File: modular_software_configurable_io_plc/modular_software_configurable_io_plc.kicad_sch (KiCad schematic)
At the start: 8 parts, among them J1 FW-14-03-G-D-085-315, J2 FW-02-03-G-D-085-315, J3 FW-02-03-G-D-085-315, J4 FW-04-03-G-D-085-315, J5 FW-04-03-G-D-085-315, J6 FW-02-03-G-D-085-315, J7 FW-02-03-G-D-085-315, J8 FW-14-03-G-D-085-315

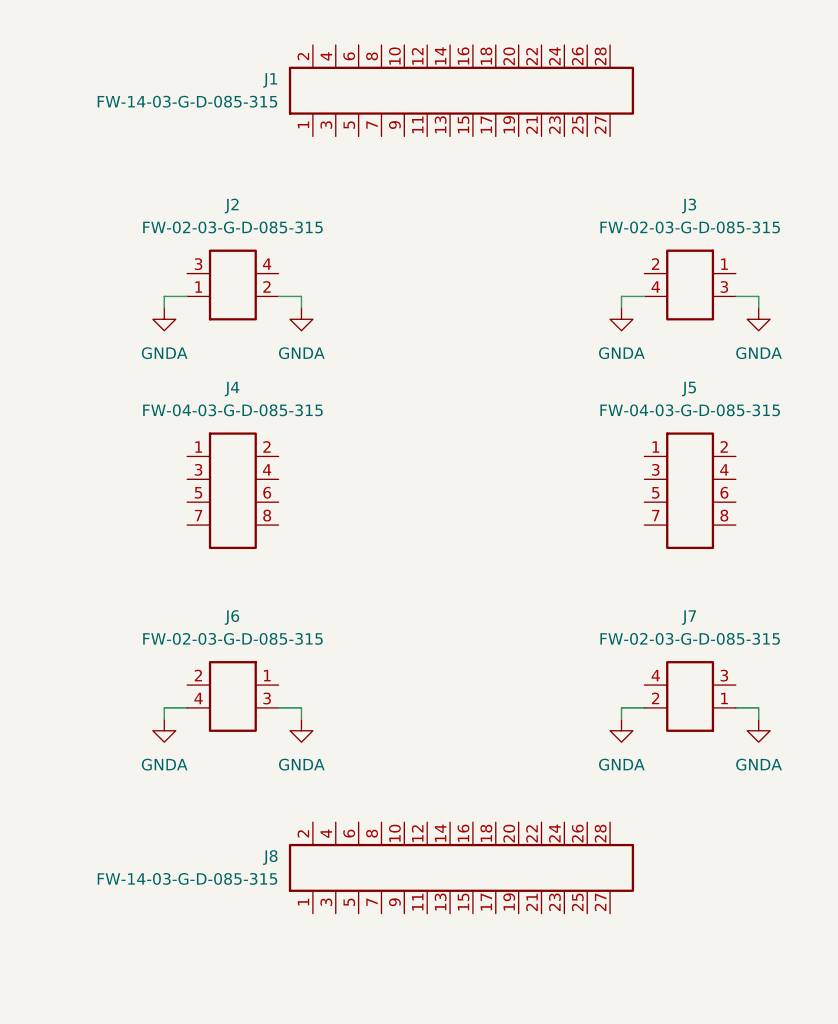
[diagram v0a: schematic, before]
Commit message: Minor updates to project files
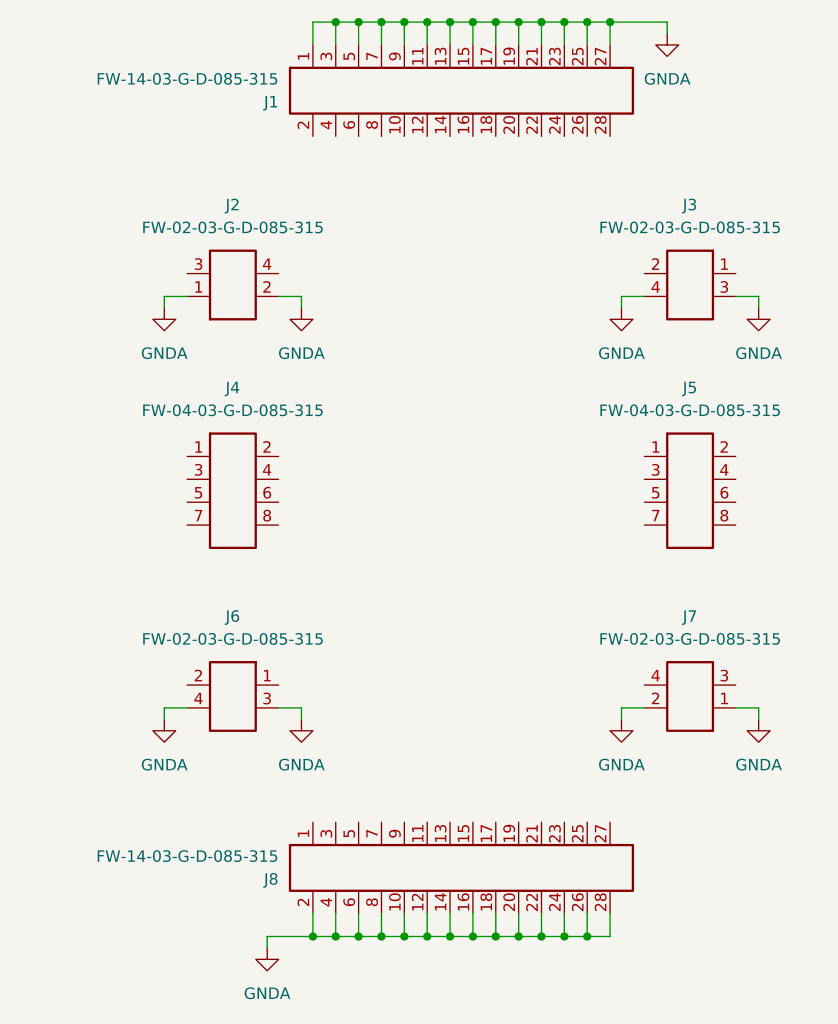
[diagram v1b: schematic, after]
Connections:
- net GNDA: now also J1.1, J1.11, J1.13, J1.15, J1.17, J1.19, J1.21, J1.23, J1.25, J1.27, J1.3, J1.5, J1.7, J1.9, J8.10, J8.12, J8.14, J8.16, J8.18, J8.2, J8.20, J8.22, J8.24, J8.26, J8.28, J8.4, J8.6, J8.8
